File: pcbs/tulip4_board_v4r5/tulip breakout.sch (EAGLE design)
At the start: 61 parts, among them IC1 MCP73831/OT, J1 CSP-USC16-TR, U1 ESP32-S3-WROOM-2-N32R8V, U2 LD29150DT33R, U3 PCM5101APW, U6 CH340C, X2 FH12-40S-0.5SH

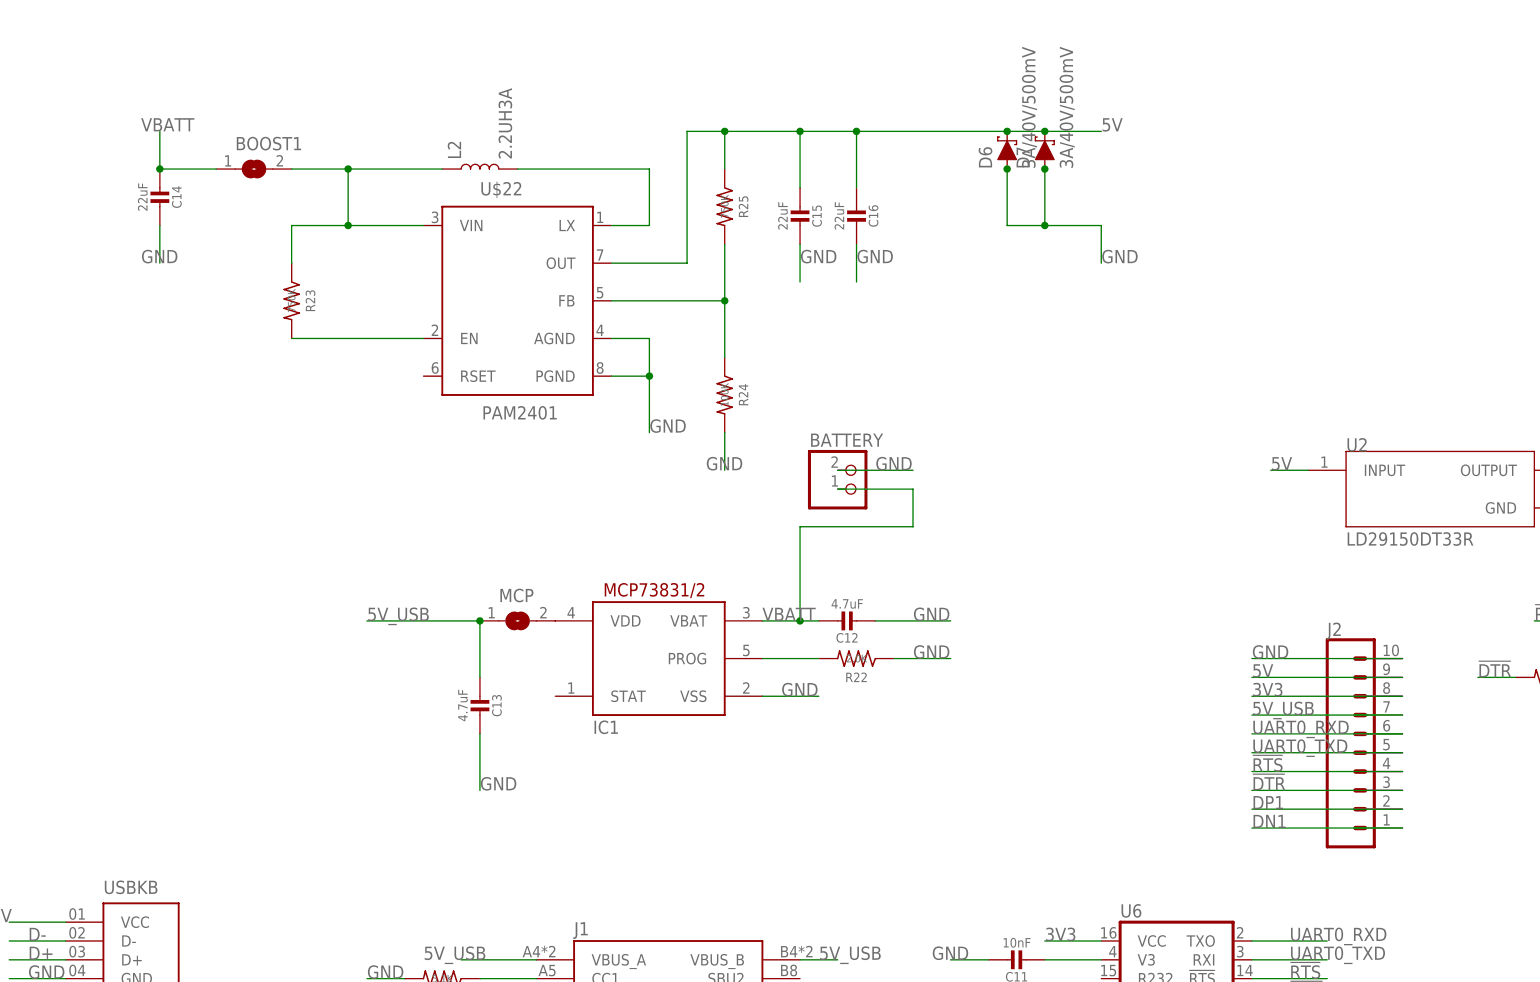
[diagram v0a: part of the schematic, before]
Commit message: .
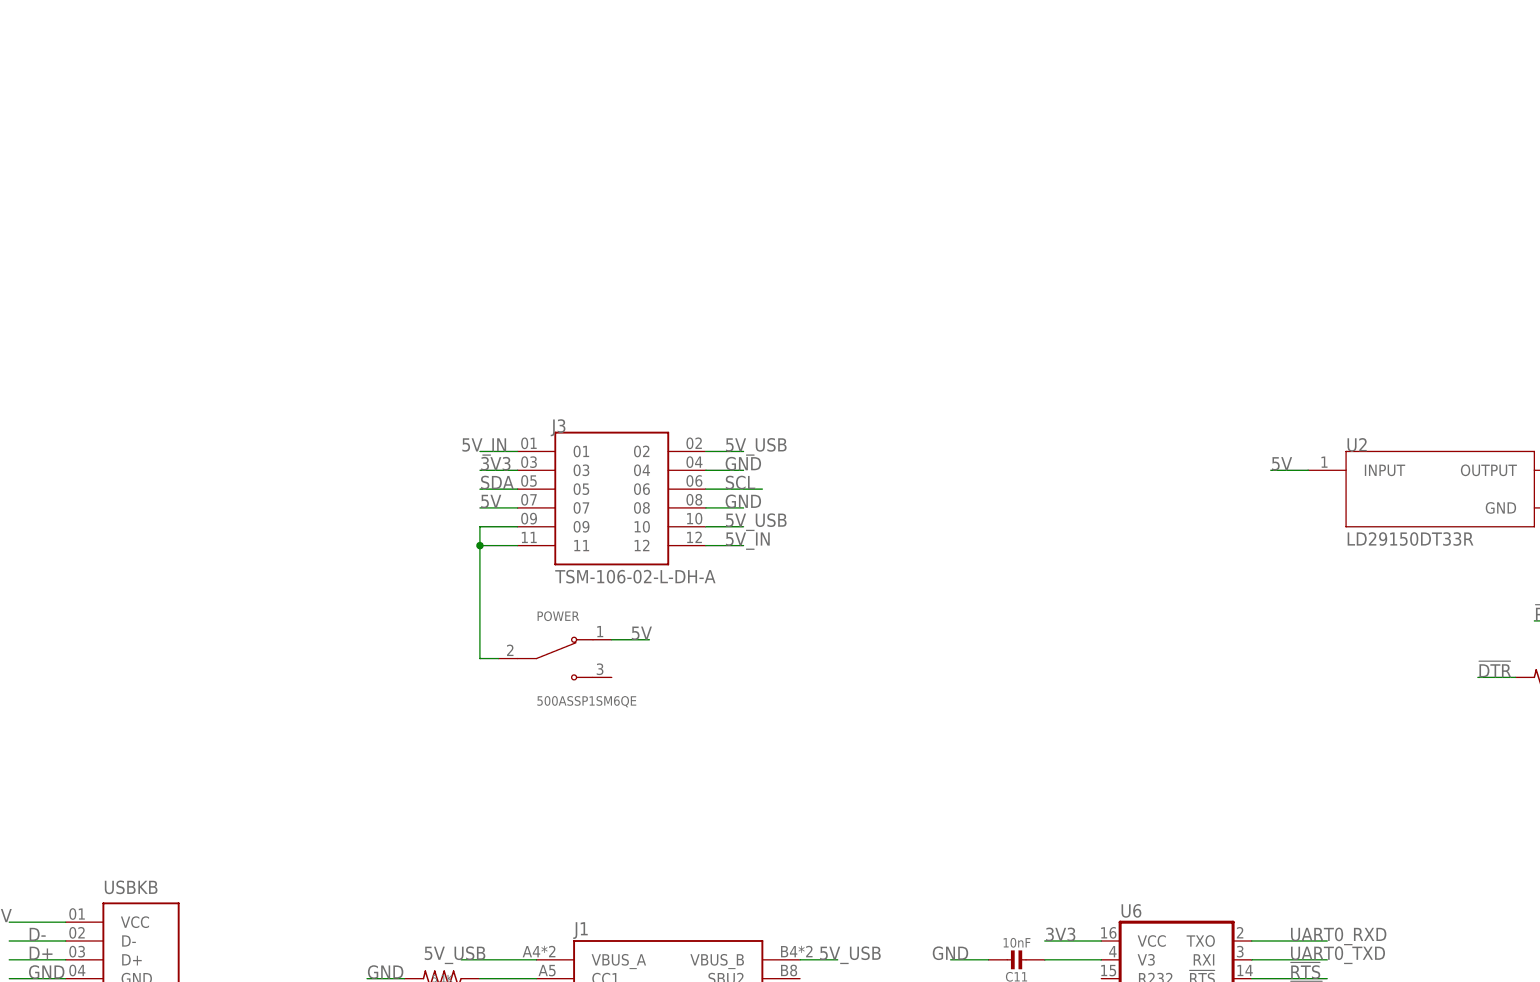
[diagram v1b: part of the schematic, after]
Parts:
- removed BATTERY: (no value), adafruit:JST_2PIN-SMT-RA
- removed BOOST1, MCP: (no value), jumper:SJW
- removed C12, C13: 4.7uF, microbuilder:CAP_CERAMIC0805-NOOUTLINE
- removed C14, C15, C16: 22uF, microbuilder:CAP_CERAMIC0805-NOOUTLINE
- removed D6, D7: 3A/40V/500mV, SparkFun-DiscreteSemi:DIODE-SCHOTTKY-B340A
- removed IC1: MCP73831/OT, adafruit:MCP73831/OT
- removed J2: (no value), SparkFun-Connectors:CONN_10"
- removed L2: 2.2UH3A, SparkFun-Coils:INDUCTOR-IFSC1515AHER2R2M01
- removed R22: 2.0K, adafruit:R-US_R0805
- removed R23, R25: 750K, adafruit:R-US_R0805
- removed R24: 100K, adafruit:R-US_R0805
- removed U$22: PAM2401, SparkFun-IC-Power:PAM2401
- added J3: TSM-106-02-L-DH-A, TSM-106-02-L-DH-A:TSM-106-02-L-DH-A
- added POWER: 500ASSP1SM6QE, 500ASSP1SM6QE:500ASSP1SM6QE
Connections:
- removed net N$17: L2.2, U$22.LX
- removed net N$19: R24.1, R25.2, U$22.FB
- removed net N$20: IC1.PROG, R22.2
- removed net N$22: R23.2, U$22.EN
- removed net N$4: IC1.VDD, MCP.2
- removed net N$6: BOOST1.2, L2.1, R23.1, U$22.VIN
- removed net VBATT: BATTERY.2, BOOST1.1, C12.1, C14.2, IC1.VBAT
- new net 5V_IN: J3.01, J3.12
- new net N$10: J3.09, J3.11, POWER.COM
- net !DTR: no longer J2.3
- net !RTS: no longer J2.4
- net 3V3: now also J3.03; no longer J2.8
- net 5V: now also J3.07, POWER.NC; no longer C15.2, C16.2, D6.C, D7.C, J2.9, R25.1, U$22.OUT
- net 5V_USB: now also J3.02, J3.10; no longer C13.2, J2.7, MCP.1
- net DN1: no longer J2.1
- net DP1: no longer J2.2
- net GND: now also J3.04, J3.08; no longer BATTERY.1, C12.2, C13.1, C14.1, C15.1, C16.1, D6.A, D7.A, IC1.VSS, J2.10, R22.1, R24.2, U$22.AGND, U$22.PGND
- net SCL: now also J3.06
- net SDA: now also J3.05
- net UART0_RXD: no longer J2.6
- net UART0_TXD: no longer J2.5
